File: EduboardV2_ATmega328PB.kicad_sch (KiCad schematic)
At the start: 14 parts, among them J1 EduboardV2 PCIE UP Board Conn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, SW1 K2-1102SP-C4SC-04, U2 ATMEGA328PB-AUR

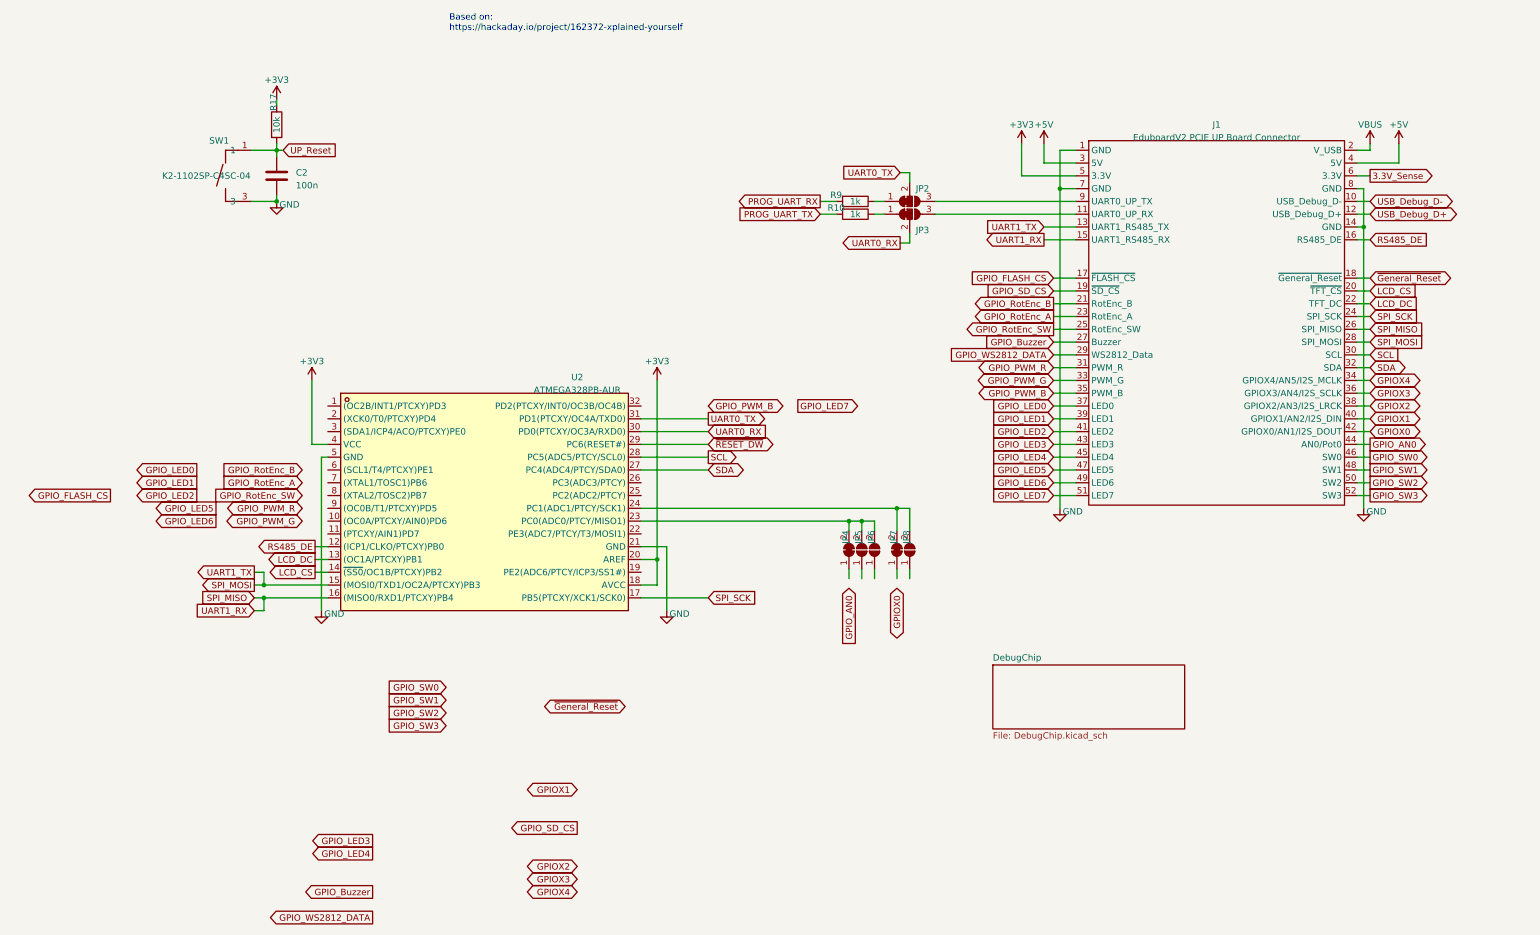
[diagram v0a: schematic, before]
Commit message: schematic done. layout done aswell. Have to check everything trice
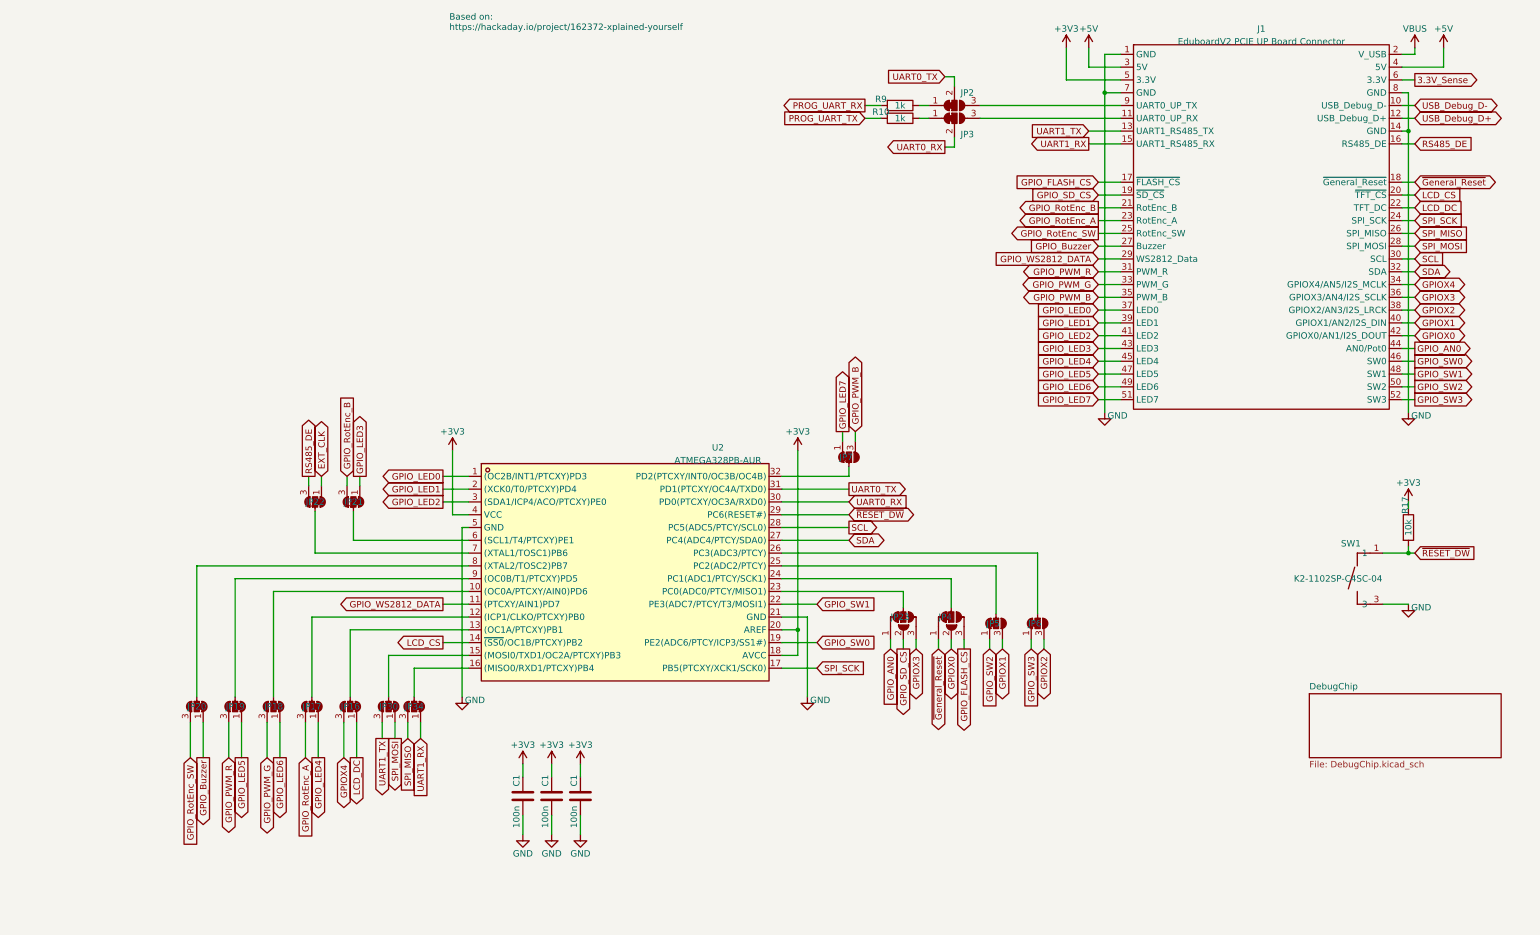
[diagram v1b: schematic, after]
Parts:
- removed C2: 100n, Capacitor_SMD:C_0603_1608Metric, symbol Device:C
- removed JP4, JP7: SolderJumper_2_Bridged, symbol Jumper:SolderJumper_2_Bridged
- removed JP5, JP6, JP8: SolderJumper_2_Open, symbol Jumper:SolderJumper_2_Open
- added C1 (x3): 100n, Capacitor_SMD:C_0402_1005Metric, symbol Device:C
- added JP16, JP17, JP18, JP19, JP20, JP21, JP22, JP30, JP34, JP5, JP6, JP7: SolderJumper_3_Bridged12, EduboardV2_kicadlib:SolderJumper_Small-3_bridged12, symbol EduboardV2_kicadlib:SolderJumper_Small_3_Bridged12
- added JP23, JP4: SolderJumper_3_Bridged12, EduboardV2_kicadlib:SolderJumper_Small-4_bridged14, symbol EduboardV2_kicadlib:SolderJumper_Small_4_Bridged14
- JP2, JP3: footprint (none) -> EduboardV2_kicadlib:SolderJumper_Small-3_bridged12
- R10, R17, R9: footprint Resistor_SMD:R_0603_1608Metric -> Resistor_SMD:R_0402_1005Metric
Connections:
- net UP_Reset is gone; now on net ~{RESET_DW}: R17.2, SW1.1, SW1.2
- net +3V3: now also C1.1, C1.1, C1.1
- net GND: now also C1.2, C1.2, C1.2
- net GPIOX0: now also JP4.2 (A)
- net GPIOX1: now also JP5.3 (B)
- net GPIOX2: now also JP6.3 (B)
- net GPIOX3: now also JP23.3 (B)
- net GPIOX4: now also JP16.3 (B)
- net GPIO_AN0: now also JP23.1 (A)
- net GPIO_Buzzer: now also JP20.1 (A)
- net GPIO_FLASH_CS: now also JP4.3 (B)
- net GPIO_LED0: now also U2.1 ((OC2B/INT1/PTCXY)PD3)
- net GPIO_LED1: now also U2.2 ((XCK0/T0/PTCXY)PD4)
- net GPIO_LED2: now also U2.3 ((SDA1/ICP4/ACO/PTCXY)PE0)
- net GPIO_LED3: now also JP21.1 (A)
- net GPIO_LED4: now also JP17.1 (A)
- net GPIO_LED5: now also JP19.1 (A)
- net GPIO_LED6: now also JP18.1 (A)
- net GPIO_LED7: now also JP7.1 (A)
- net GPIO_PWM_B: now also JP7.3 (B)
- net GPIO_PWM_G: now also JP18.3 (B)
- net GPIO_PWM_R: now also JP19.3 (B)
- net GPIO_RotEnc_A: now also JP17.3 (B)
- net GPIO_RotEnc_B: now also JP21.3 (B)
- net GPIO_RotEnc_SW: now also JP20.3 (B)
- net GPIO_SD_CS: now also JP23.2 (A)
- net GPIO_SW0: now also U2.19 (PE2(ADC6/PTCY/ICP3/SS1#))
- net GPIO_SW1: now also U2.22 (PE3(ADC7/PTCY/T3/MOSI1))
- net GPIO_SW2: now also JP5.1 (A)
- net GPIO_SW3: now also JP6.1 (A)
- net GPIO_WS2812_DATA: now also U2.11 ((PTCXY/AIN1)PD7)
- net LCD_DC: now also JP16.1 (A); no longer U2.13 ((OC1A/PTCXY)PB1)
- net RS485_DE: now also JP22.3 (B); no longer U2.12 ((ICP1/CLKO/PTCXY)PB0)
- net SPI_MISO: now also JP34.3 (B); no longer J1.15 (UART1_RS485_RX), U2.16 ((MISO0/RXD1/PTCXY)PB4)
- net SPI_MOSI: now also JP30.1 (A); no longer J1.13 (UART1_RS485_TX), U2.15 ((MOSI0/TXD1/OC2A/PTCXY)PB3)
- net ~{General_Reset}: now also JP4.1 (A)
- net at U2.24 (PC1(ADC1/PTCY/SCK1)): now also JP4.4 (C)
- net at U2.23 (PC0(ADC0/PTCY/MISO1)): now also JP23.4 (C)
- net at U2.10 ((OC0A/PTCXY/AIN0)PD6): now also JP18.2 (C)
- net at U2.25 (PC2(ADC2/PTCY)): now also JP5.2 (C)
- net at U2.26 (PC3(ADC3/PTCY)): now also JP6.2 (C)
- net at U2.32 (PD2(PTCXY/INT0/OC3B/OC4B)): now also JP7.2 (C)
- net at U2.6 ((SCL1/T4/PTCXY)PE1): now also JP21.2 (C)
- net at U2.7 ((XTAL1/TOSC1)PB6): now also JP22.2 (C)
- net at U2.8 ((XTAL2/TOSC2)PB7): now also JP20.2 (C)
- net at U2.9 ((OC0B/T1/PTCXY)PD5): now also JP19.2 (C)
- new net: JP30.2 (C), U2.15 ((MOSI0/TXD1/OC2A/PTCXY)PB3)
- new net: JP17.2 (C), U2.12 ((ICP1/CLKO/PTCXY)PB0)
- new net: JP16.2 (C), U2.13 ((OC1A/PTCXY)PB1)
- new net: JP34.2 (C), U2.16 ((MISO0/RXD1/PTCXY)PB4)
- new net EXT_CLK: JP22.1 (A)
- new net UART1_RX: J1.15 (UART1_RS485_RX), JP34.1 (A)
- new net UART1_TX: J1.13 (UART1_RS485_TX), JP30.3 (B)
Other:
- moved on the sheet: J1, JP2, JP3, R10, R17, R9, SW1, U2
